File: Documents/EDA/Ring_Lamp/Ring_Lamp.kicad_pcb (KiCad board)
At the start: 2 copper layers, 90.1 x 61.2 mm, 22 parts, among them J101 Conn_01x02, M2.5 MountingHole

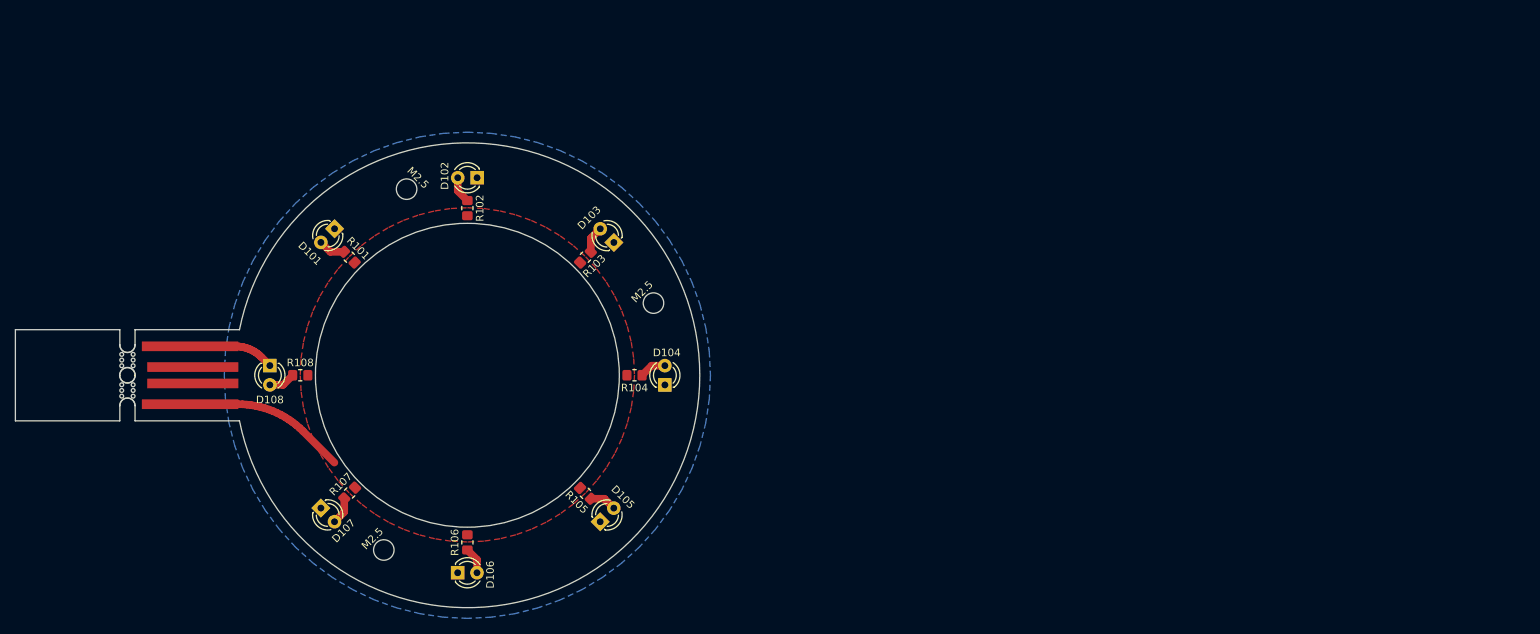
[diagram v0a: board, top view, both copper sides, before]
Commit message: ring light
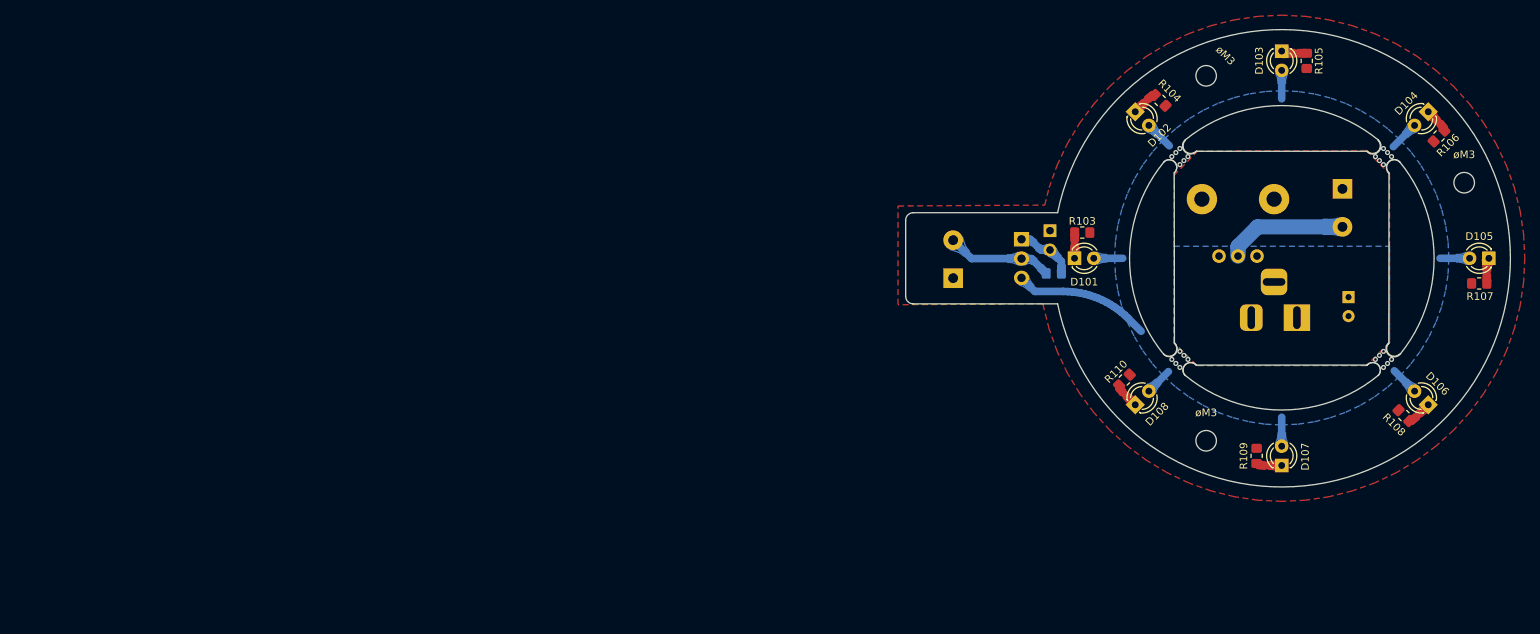
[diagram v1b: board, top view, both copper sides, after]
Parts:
- removed M2.5 (x3): MountingHole, MountingHole:MountingHole_2.7mm_M2.5
- removed the mouse-bite-2mm-slot at (86.8, 136.4)
- removed the mouse-bite-2mm-slot at (86.8, 140.4)
- added C101: 100u, Capacitor_THT:CP_Radial_D5.0mm_P2.50mm, B.Cu at (247.5, 128.1)
- added J102: Barrel_Jack, Connector_BarrelJack:BarrelJack_Horizontal, B.Cu at (240.7, 130.8)
- added J103: RING_V_LED, TerminalBlock_Phoenix:TerminalBlock_Phoenix_MKDS-1,5-2_1x02_P5.00mm_Horizontal, B.Cu at (195.4, 125.6)
- added J104: ENABLE, Connector_PinHeader_2.54mm:PinHeader_1x02_P2.54mm_Vertical, B.Cu at (208.2, 119.3)
- added Q101: Q_NMOS_GDS, Package_TO_SOT_THT:TO-220-3_Vertical, B.Cu at (204.4, 120.5)
- added R109: 100, Resistor_SMD:R_0805_2012Metric_Pad1.20x1.40mm_HandSolder, F.Cu at (235.4, 149.0)
- added R110: 100, Resistor_SMD:R_0805_2012Metric_Pad1.20x1.40mm_HandSolder, F.Cu at (218.0, 139.0)
- added mouse-bite-2mm-slot: VAL**, Panelization:mouse-bite-2mm-slot, F.Cu at (252.1, 136.3)
- added mouse-bite-2mm-slot: VAL**, Panelization:mouse-bite-2mm-slot, F.Cu at (225.3, 109.6)
- added mouse-bite-2mm-slot: VAL**, Panelization:mouse-bite-2mm-slot, F.Cu at (225.3, 136.3)
- added mouse-bite-2mm-slot: VAL**, Panelization:mouse-bite-2mm-slot, F.Cu at (252.1, 109.6)
- added øM3: MountingHole, MountingHole:MountingHole_2.7mm_M2.5, F.Cu at (228.8, 147.0)
- added øM3: MountingHole, MountingHole:MountingHole_2.7mm_M2.5, F.Cu at (262.7, 113.0)
- added øM3: MountingHole, MountingHole:MountingHole_2.7mm_M2.5, F.Cu at (228.8, 99.0)
- J101: value Conn_01x02 -> CTRL_V_LED; footprint footprints:USBA_Pads -> TerminalBlock_Phoenix:TerminalBlock_Phoenix_MKDS-1,5-2_1x02_P5.00mm_Horizontal; moved to B.Cu
- R101: value 100 -> 10k; moved to B.Cu
- R102: value 100 -> 10k; footprint Resistor_SMD:R_0805_2012Metric_Pad1.20x1.40mm_HandSolder -> Potentiometer_THT:Potentiometer_Alps_RK09L_Single_Vertical; moved to B.Cu
- moved J101 153.7 mm to (246.7, 113.8), turned to 270 degrees
- moved R107 151.2 mm to (264.7, 126.3), turned to 0 degrees
- moved R108 145.4 mm to (254.8, 143.7), turned to 315 degrees
- moved R106 138.6 mm to (259.4, 106.9), turned to 45 degrees
- moved D106 129.7 mm to (258.0, 142.3), turned to 135 degrees
- moved D107 126.6 mm to (238.7, 150.3), turned to 90 degrees
- moved D105 122.0 mm to (266.0, 123.0), turned to 180 degrees
- moved D108 114.0 mm to (219.4, 142.3), turned to 45 degrees
- moved R105 110.7 mm to (242.0, 97.0), turned to 90 degrees
- moved D104 106.7 mm to (258.0, 103.7), turned to 225 degrees
- moved R102 99.1 mm to (230.4, 122.7), turned to 90 degrees
- moved D101 97.5 mm to (211.4, 123.0), turned to 0 degrees
- moved R101 92.8 mm to (208.7, 125.0), turned to 0 degrees
- moved D103 91.5 mm to (238.7, 95.7), turned to 270 degrees
- moved D102 87.1 mm to (219.4, 103.7), turned to 315 degrees
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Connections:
- D101 pad 1: GND -> Net-(D101-Pad1)
- D101 pad 2: Net-(D101-Pad2) -> /LED_BUS
- D102 pad 1: GND -> Net-(D102-Pad1)
- D102 pad 2: Net-(D102-Pad2) -> /LED_BUS
- D103 pad 1: GND -> Net-(D103-Pad1)
- D103 pad 2: Net-(D103-Pad2) -> /LED_BUS
- D104 pad 1: GND -> Net-(D104-Pad1)
- D104 pad 2: Net-(D104-Pad2) -> /LED_BUS
- D105 pad 1: GND -> Net-(D105-Pad1)
- D105 pad 2: Net-(D105-Pad2) -> /LED_BUS
- D106 pad 1: GND -> Net-(D106-Pad1)
- D106 pad 2: Net-(D106-Pad2) -> /LED_BUS
- D107 pad 1: GND -> Net-(D107-Pad1)
- D107 pad 2: Net-(D107-Pad2) -> /LED_BUS
- D108 pad 1: GND -> Net-(D108-Pad1)
- D108 pad 2: Net-(D108-Pad2) -> /LED_BUS
- J101 pad 1: +5V -> GND
- J101 pad 2: GND -> /V_LED
- R101 pad 1: Net-(D101-Pad2) -> /V_LED
- R101 pad 2: +5V -> /ENABLE
- R102 pad 1: Net-(D102-Pad2) -> VDD
- R102 pad 2: +5V -> /V_LED
- R103 pad 1: Net-(D103-Pad2) -> GND
- R103 pad 2: +5V -> Net-(D101-Pad1)
- R104 pad 1: Net-(D104-Pad2) -> GND
- R104 pad 2: +5V -> Net-(D102-Pad1)
- R105 pad 1: Net-(D105-Pad2) -> GND
- R105 pad 2: +5V -> Net-(D103-Pad1)
- R106 pad 1: Net-(D106-Pad2) -> GND
- R106 pad 2: +5V -> Net-(D104-Pad1)
- R107 pad 1: Net-(D107-Pad2) -> GND
- R107 pad 2: +5V -> Net-(D105-Pad1)
- R108 pad 1: Net-(D108-Pad2) -> GND
- R108 pad 2: +5V -> Net-(D106-Pad1)
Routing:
- net /LED_BUS: track 0.00 -> 48.6 mm
- net /V_LED: track 0.00 -> 30.2 mm
- net +5V: track 21.7 -> 0.00 mm
- net GND: track 11.3 -> 0.00 mm
- net /ENABLE: track 0.00 -> 8.09 mm
- net Net-(D107-Pad2): track 3.60 -> 0.00 mm
- net Net-(D105-Pad2): track 3.54 -> 0.00 mm
- net Net-(D103-Pad2): track 3.54 -> 0.00 mm
- net Net-(D101-Pad2): track 3.54 -> 0.00 mm
- net Net-(D106-Pad2): track 3.52 -> 0.00 mm
- net Net-(D104-Pad2): track 3.52 -> 0.00 mm
- net Net-(D108-Pad2): track 3.52 -> 0.00 mm
- net Net-(D102-Pad2): track 3.52 -> 0.00 mm
- net Net-(D102-Pad1): track 0.00 -> 3.49 mm
- net Net-(D108-Pad1): track 0.00 -> 3.44 mm
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- added copper zone on B.Cu, net /LED_BUS
- added copper zone on F.Cu, net GND
- added copper zone on B.Cu, net VDD
- removed copper zone on F.Cu, net +5V
- removed copper zone on B.Cu, net GND
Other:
- board size 90.1 x 61.2 mm -> 79.6 x 60.2 mm
